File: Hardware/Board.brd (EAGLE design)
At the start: 46 x 35 mm, 103 parts, among them IC1 BQ25180YBGR_BQ25180YBGR, IC2 RT6160AWSC_RT6160AWSC, IC3 BMA423_BMA423, IC4 DRV2605YZFR, J1 TC2030-IDC_TC2030-IDC, J3 503480-2400, J4 KH-TYPE-C-16P, Q1 20V/4.2A/52mΩ/1.4W, Q3 ESP32_C6_LIBRARY_6_SI1308EDL-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, U3 MAX17048G+T10, X1 32MHz, X2 32.768kHz

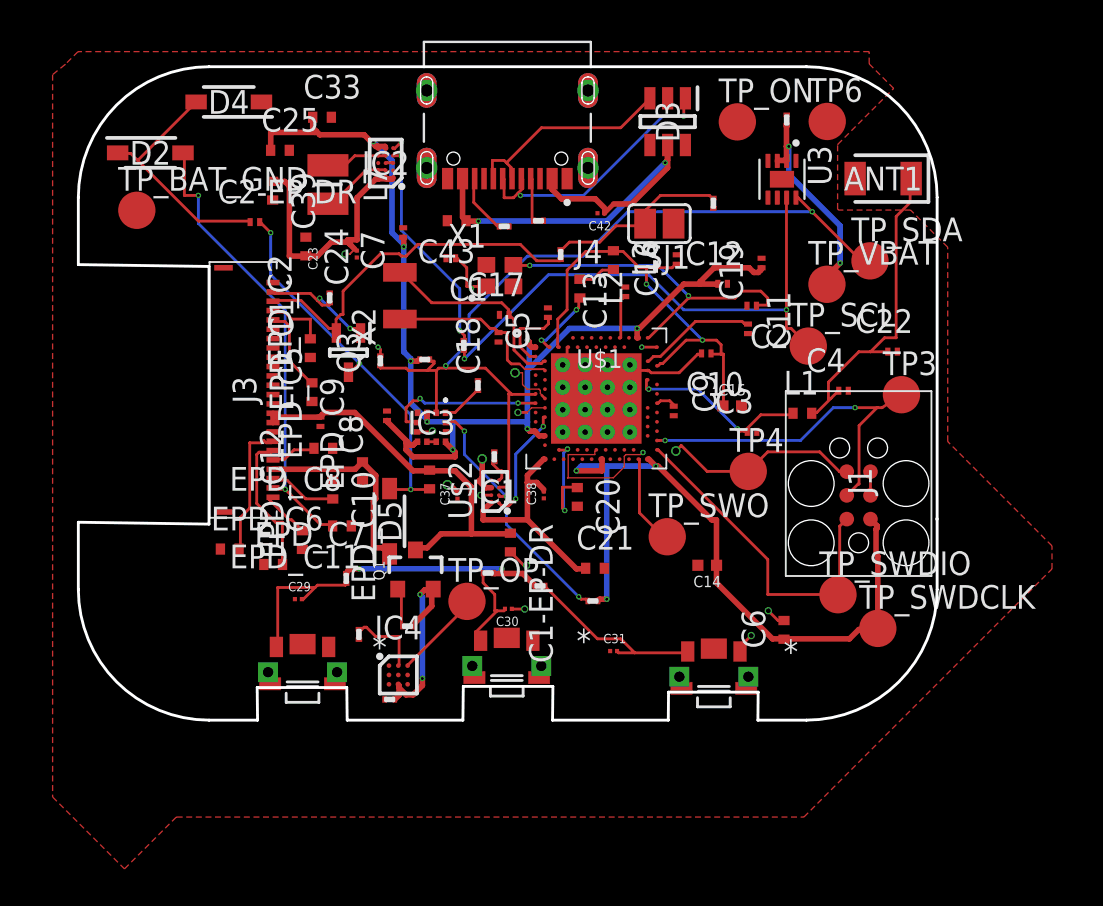
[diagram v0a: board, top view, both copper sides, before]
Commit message: Add files via upload
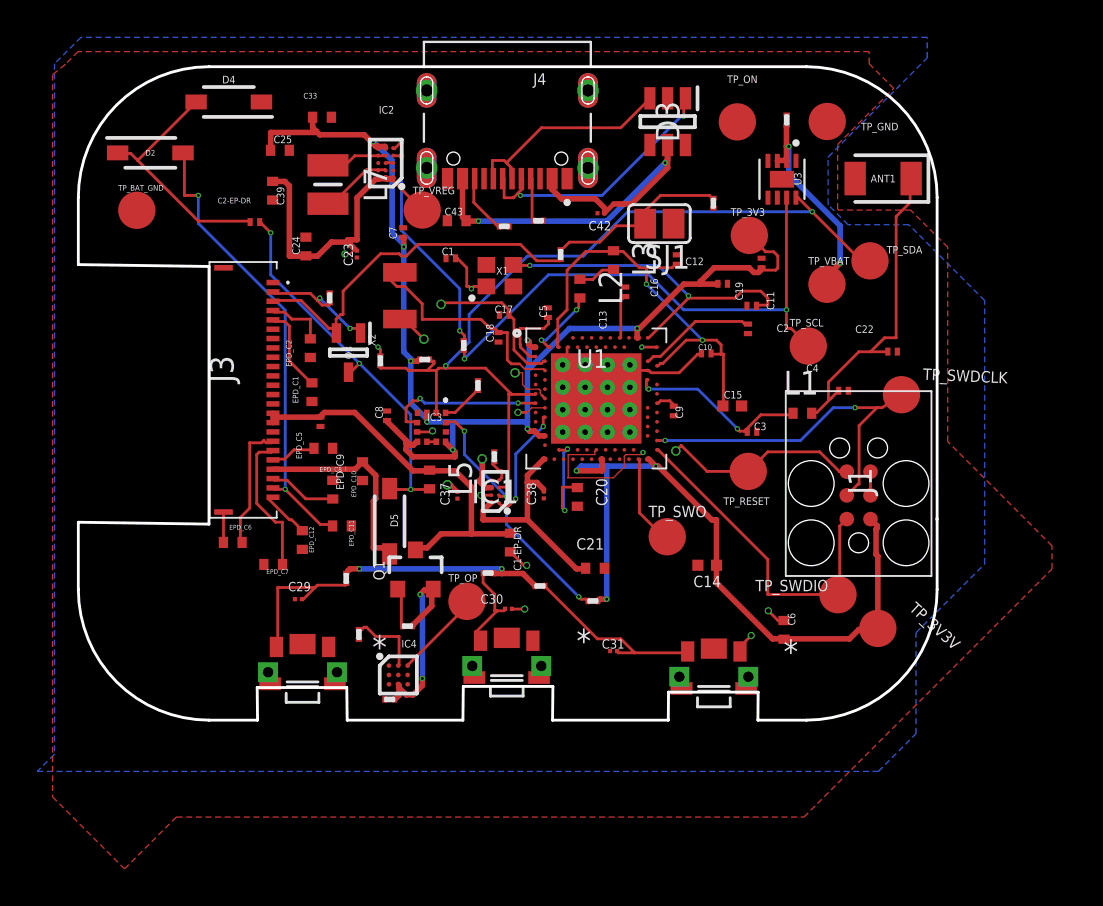
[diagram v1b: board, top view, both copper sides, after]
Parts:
- removed TP3: HECTOR_WATCH_1_TPTP20R, InkTime_v5:HECTOR_WATCH_1_TP20R
- added TP_3V3, TP_3V3V, TP_VREG: HECTOR_WATCH_1_TPTP20R, InkTime_v5:HECTOR_WATCH_1_TP20R
- C9: value 820pF -> 820pF N.C.
- L5: value (none) -> 68uH
- moved TP_SWDCLK 12.6 mm to (20.9, -0.80)
- moved EPD_C6 0.39 mm to (-14.9, -8.71)
- renumbered TP4 to TP_RESET, TP6 to TP_GND, U$1 to U1, U$2 to L5
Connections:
- removed net N$9: C18.2, U1.P$F2, X2.1
- new net N$2: C18.2, U1.P$F2, X2.2
- net 3V3/2.4A: now also TP_3V3.TP, TP_3V3V.TP; no longer TP_SWDCLK.TP
- net N$10: now also X2.1; no longer X2.2
- net SWDCLK: now also TP_SWDCLK.TP; no longer TP3.TP
- net VREG: now also TP_VREG.TP
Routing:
- net N$2: track 0.00 -> 12.4 mm
- net N$9: track 9.78 -> 0.00 mm
- net 3V3/2.4A: track 105.1 -> 108.7 mm
- net VREG: track 35.9 -> 38.2 mm
- net GND: track 43.7 -> 45.3 mm
- net N$10: track 10.9 -> 12.1 mm, vias 0 -> 2
- added copper zone on layer 16, net GND

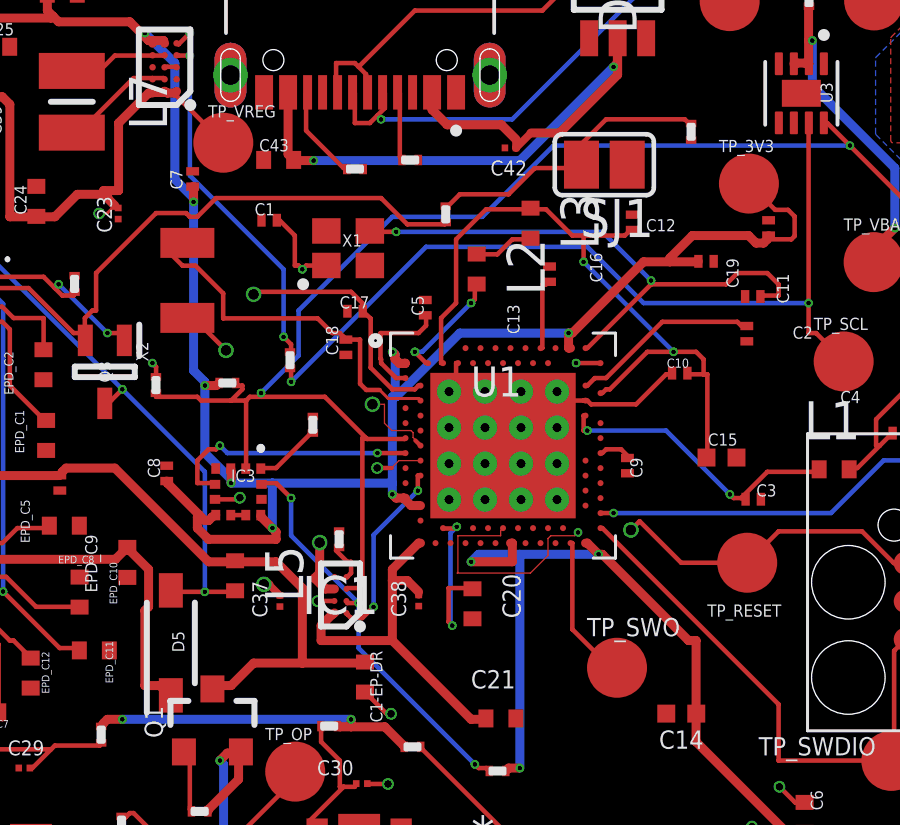
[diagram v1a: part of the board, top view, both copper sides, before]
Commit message: Update Board.brd
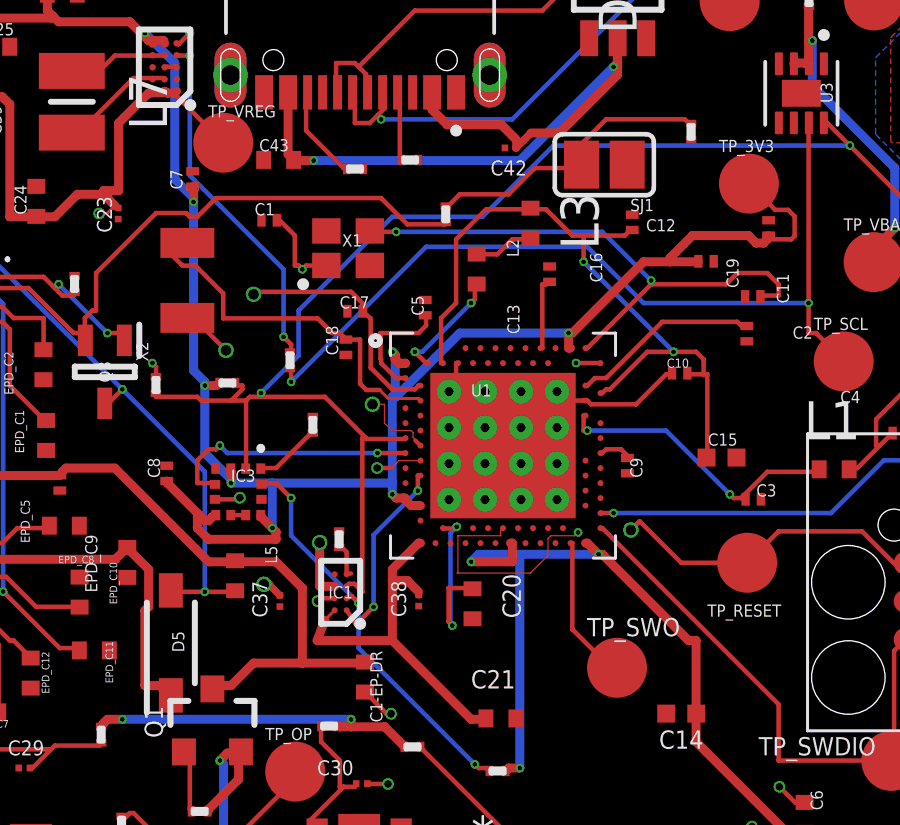
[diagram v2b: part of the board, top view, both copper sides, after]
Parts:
- moved IC1 0.09 mm to (-0.85, -5.89)
